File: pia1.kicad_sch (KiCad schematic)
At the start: 38 parts, among them IC20 MC14529B, IC24 74LS244N, IC25 LM393P, IC26 MC6821, IC31 74LS02N, U2 GAL22V10

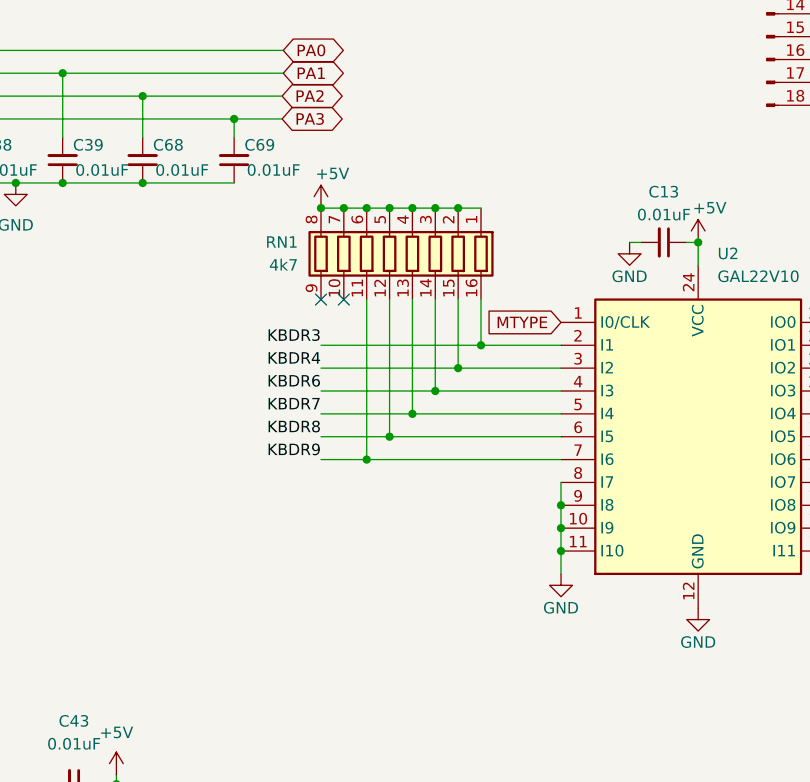
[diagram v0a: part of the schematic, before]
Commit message: refresh BOM
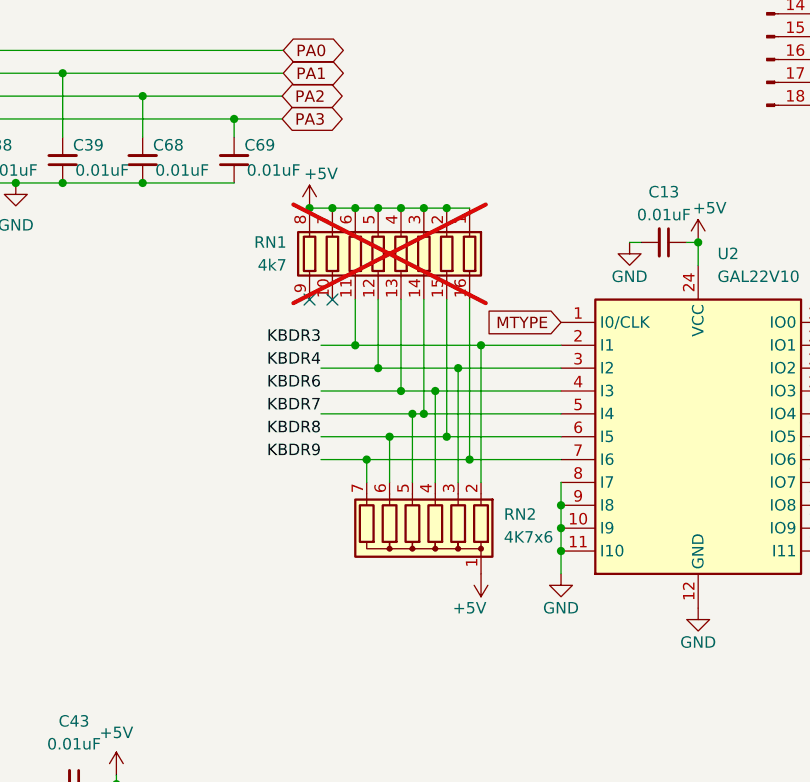
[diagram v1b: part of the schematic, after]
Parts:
- added RN2: 4K7x6, Resistor_THT:R_Array_SIP7, symbol Device:R_Network06
- C30, C31, C32, C33: LCSC (none) -> C1729
- IC24: LCSC (none) -> C22374098
- IC25: LCSC (none) -> C5209
- IC31: LCSC (none) -> C22374091; SA2120 Sheet 1 (spare) -> (none)
- RN1: now not fitted
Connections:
- net +5V: now also RN2.1 (common)
- net KBDR3: now also RN1.11 (R6.2), RN2.2 (R1); no longer RN1.16 (R1.2)
- net KBDR4: now also RN1.12 (R5.2), RN2.3 (R2); no longer RN1.15 (R2.2)
- net KBDR6: now also RN1.13 (R4.2), RN2.4 (R3); no longer RN1.14 (R3.2)
- net KBDR7: now also RN1.14 (R3.2), RN2.5 (R4); no longer RN1.13 (R4.2)
- net KBDR8: now also RN1.15 (R2.2), RN2.6 (R5); no longer RN1.12 (R5.2)
- net KBDR9: now also RN1.16 (R1.2), RN2.7 (R6); no longer RN1.11 (R6.2)

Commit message: align versions
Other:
- title: (none) -> Dragon CPU UK Revised
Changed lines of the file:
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@@
 	(paper "A3")
 	(title_block
-		(date "2023-05-25")
-		(rev "3.0")
+		(title "Dragon CPU UK Revised")
+		(date "2025-10-05")
+		(rev "3.3")
+		(comment 1 "Redesign by Julian Brown")
 		(comment 2 "Reposition dram and buffer")
 	)
